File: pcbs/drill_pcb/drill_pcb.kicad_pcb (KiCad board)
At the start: 2 copper layers, 109 x 112 mm, 27 parts, among them J1 24V IN, J10 WEIGHT SENSOR, J11 STEPPER STORAGE, J2 DC MOTOR 24 V, J3 DC MOTOR UART, J4 ENCODER VERTICAL DRIVE, J5 LIMIT SENSOR TOP, J6 HEIGHT SENSOR, J7 STEPPER VERTICAL DRIVE, J8 ENCODER STORAGE, J9 LIMIT SENSOR BOTTOM, U1 ESP32-DevKitC, U2 LM3940

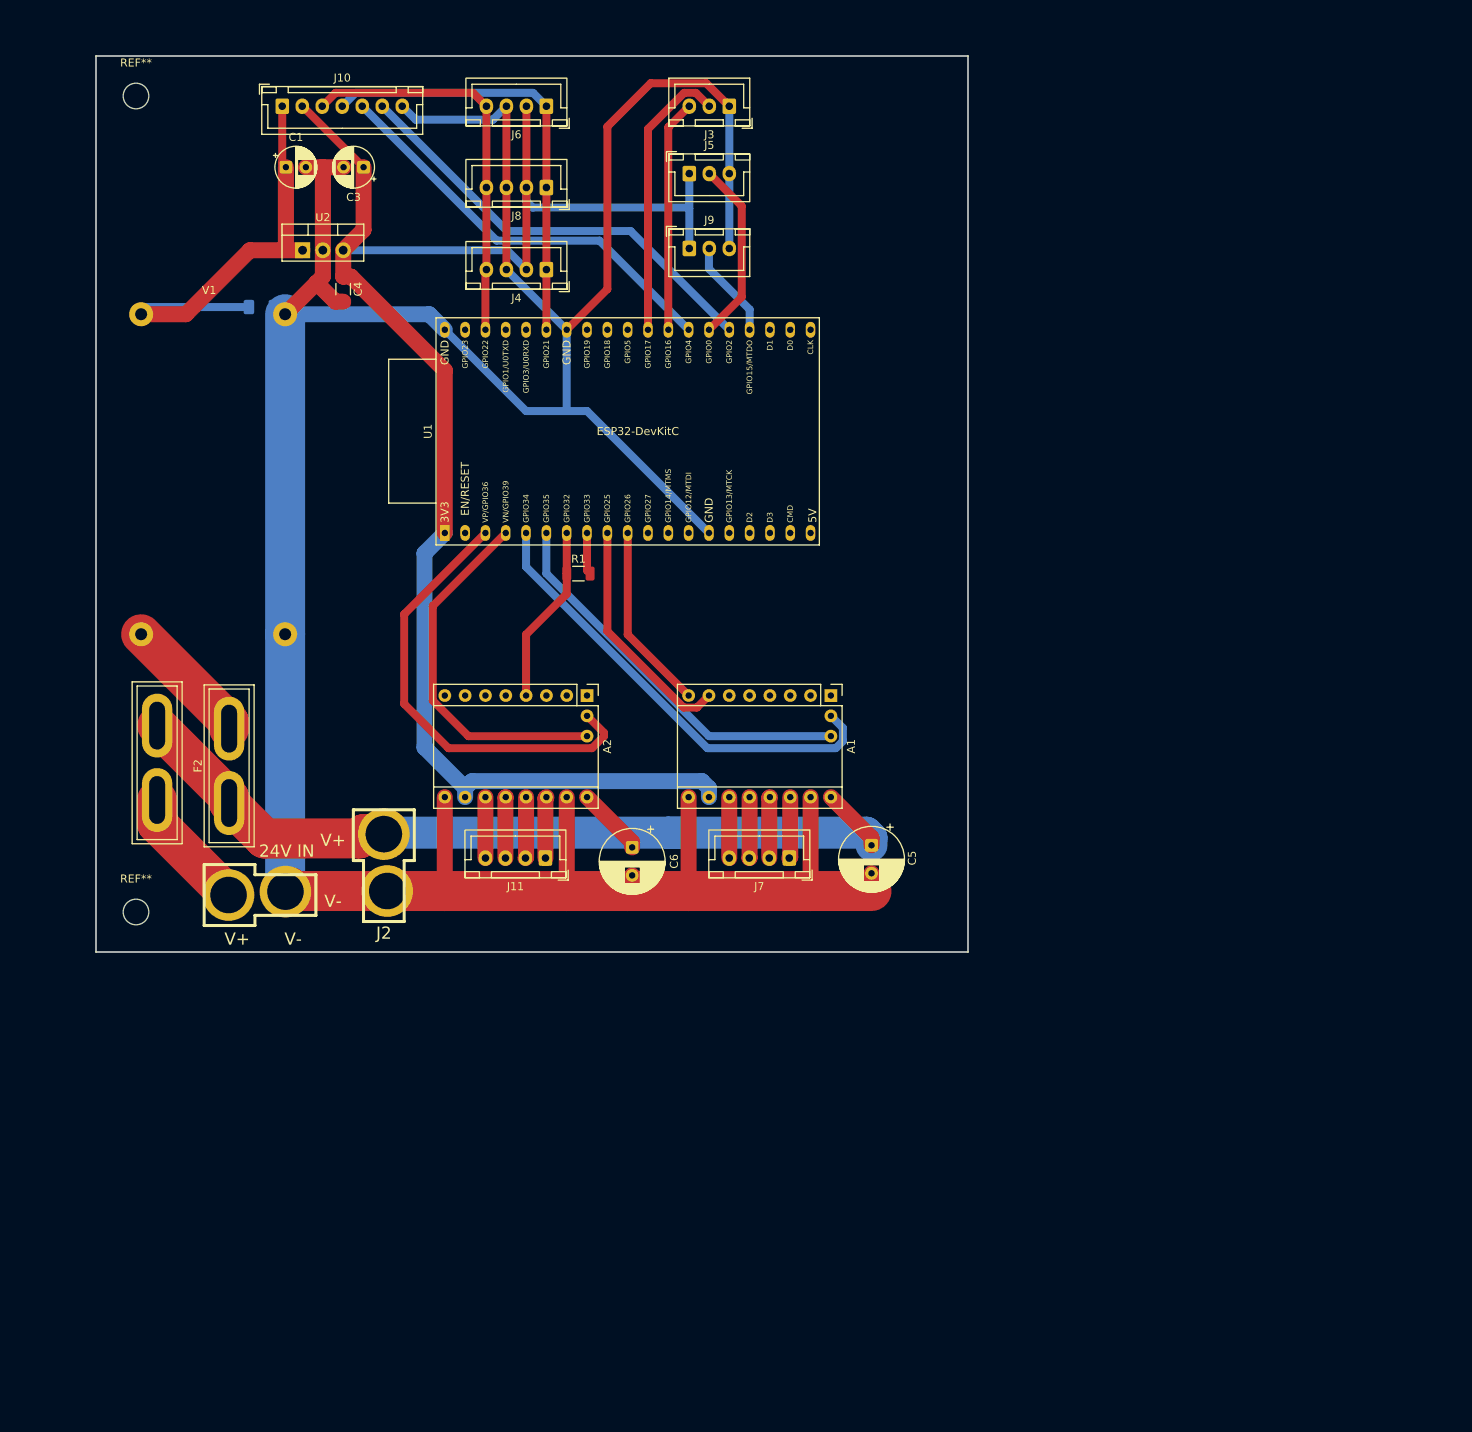
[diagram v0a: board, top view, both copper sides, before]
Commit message: PCB should be fully complete now. Somebody pls review it :(
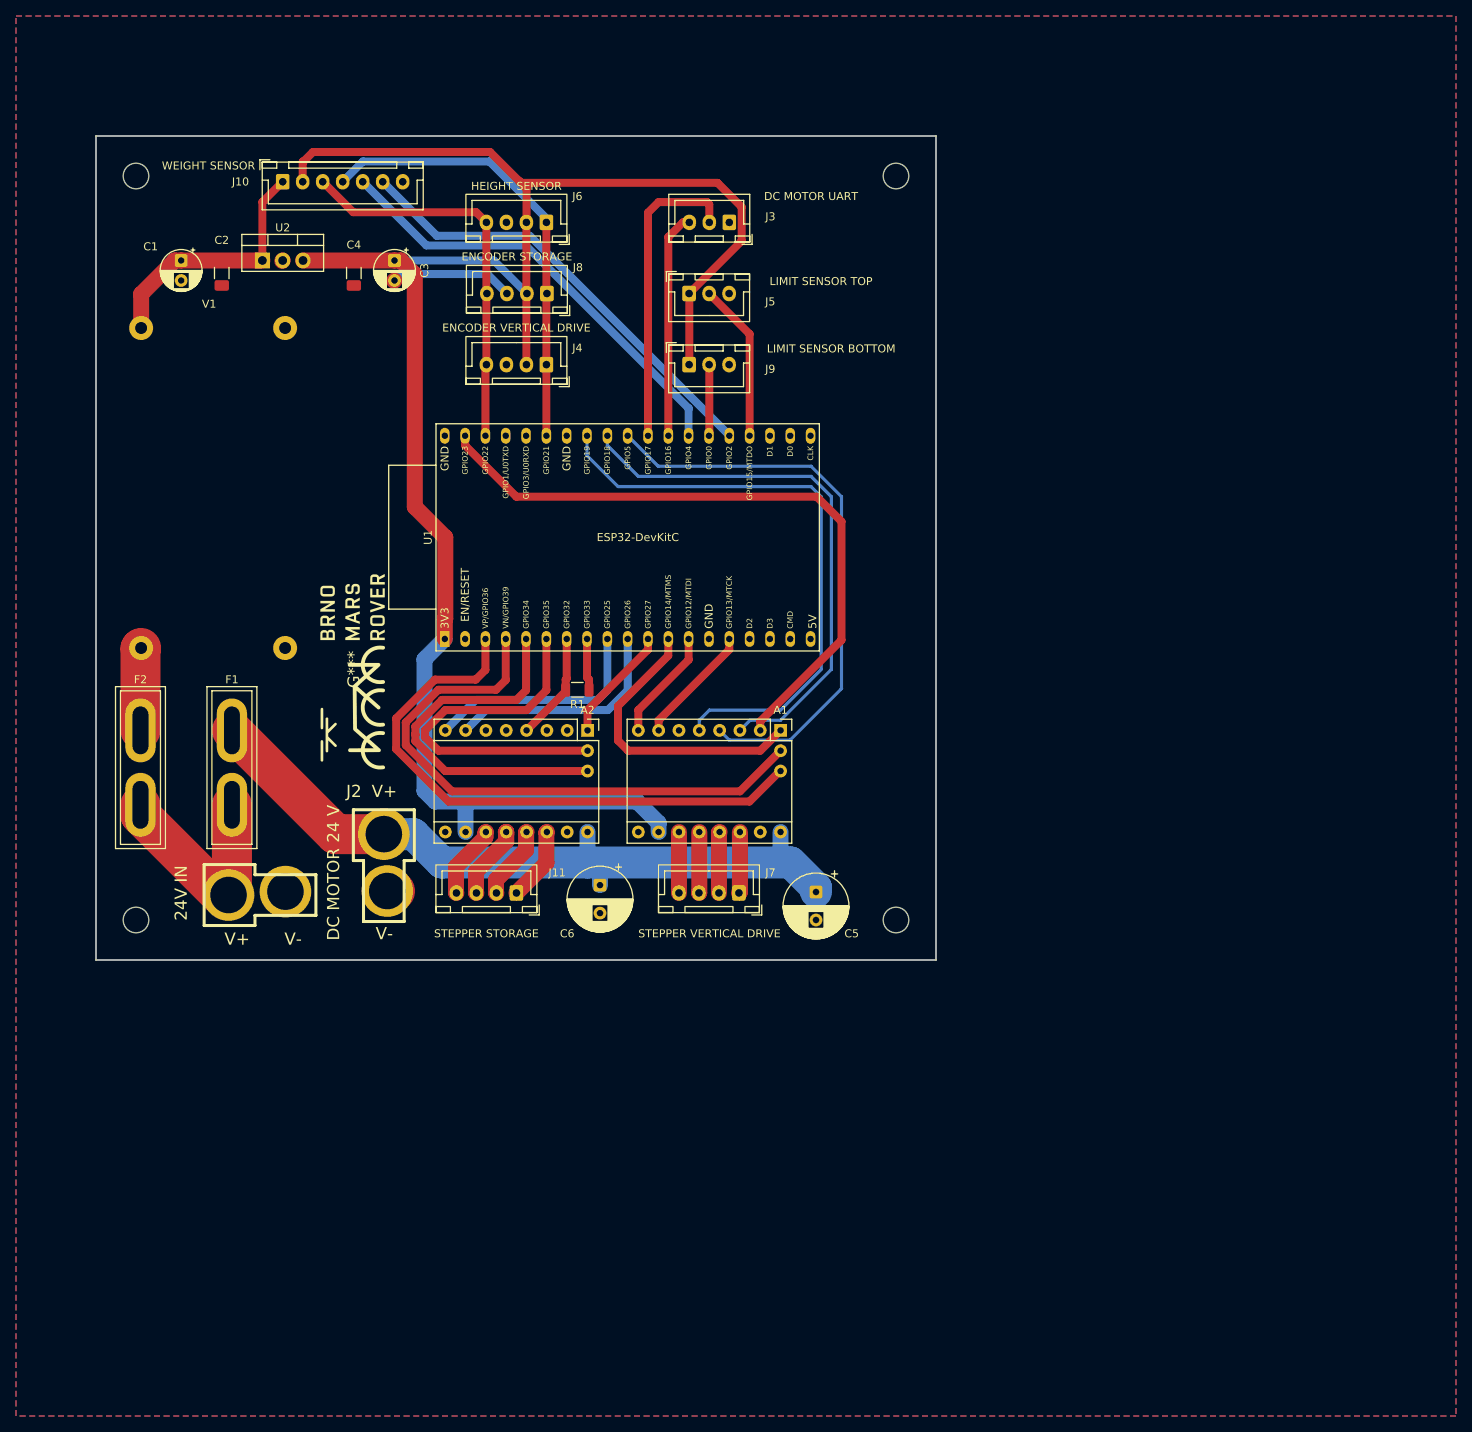
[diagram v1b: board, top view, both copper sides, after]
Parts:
- removed the REF** at (35.0, 137.0)
- removed the REF** at (35.0, 35.0)
- added G***: LOGO, logo:logo, F.Cu at (62.2, 106.7)
- added REF**: MountingHole_3.2mm_M3, MountingHole:MountingHole_3.2mm_M3, F.Cu at (35.0, 45.0)
- added REF**: MountingHole_3.2mm_M3, MountingHole:MountingHole_3.2mm_M3, F.Cu at (35.0, 138.0)
- added REF**: MountingHole_3.2mm_M3, MountingHole:MountingHole_3.2mm_M3, F.Cu at (130.0, 138.0)
- added REF**: MountingHole_3.2mm_M3, MountingHole:MountingHole_3.2mm_M3, F.Cu at (130.0, 45.0)
- C2: moved to F.Cu
- moved C1 17.5 mm to (40.6, 55.6), turned to -90 degrees
- moved J5 15.0 mm to (104.1, 59.7)
- moved R1 14.5 mm to (90.2, 109.2)
- moved J9 14.5 mm to (104.1, 68.6)
- moved J3 14.5 mm to (109.2, 50.8)
- moved J6 14.5 mm to (86.3, 50.8)
- moved J8 13.3 mm to (86.4, 59.7)
- moved U1 13.2 mm to (73.6, 102.9)
- moved C3 12.3 mm to (67.3, 55.6), turned to -90 degrees
- moved J4 11.9 mm to (86.3, 68.6)
- moved F2 11.1 mm to (35.6, 123.6)
- moved J10 9.44 mm to (53.3, 45.7)
- moved F1 9.37 mm to (47.0, 123.6)
- moved C5 9.07 mm to (120.0, 134.5)
- moved A1 7.65 mm to (115.6, 114.3)
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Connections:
- F2 pad 1: +24V -> Net-(J1-Pin_1)
- U1 pad 10: DRVR_VERT_DIR -> DRVR_STORAGE_STEP
- U1 pad 11: DRVR_VERT_ENABLE -> DRVR_STORAGE_ENABLE
- U1 pad 12: DRVR_STORAGE_ENABLE -> DRVR_VERT_ENABLE
- U1 pad 13: DRVR_STORAGE_DIR -> DRVR_VERT_DIR
- U1 pad 15: DRVR_STORAGE_STEP -> DRVR_VERT_STEP
- U1 pad 23: LIMIT_SENSOR_BOTTOM -> LIMIT_SENSOR_TOP
- U1 pad 25: LIMIT_SENSOR_TOP -> LIMIT_SENSOR_BOTTOM
- U1 pad 3: DRVR_STORAGE_0 -> DRVR_VERT_DIAG1
- U1 pad 4: DRVR_STORAGE_1 -> DRVR_VERT_DIAG0
- U1 pad 5: DRVR_VERT_DIAG0 -> DRVR_STORAGE_1
- U1 pad 6: DRVR_VERT_DIAG1 -> DRVR_STORAGE_0
- U1 pad 9: DRVR_VERT_STEP -> DRVR_STORAGE_DIR
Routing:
- net GND: track 416.0 -> 16.6 mm
- net VSPI_MOSI: track 0.00 -> 82.5 mm
- net VSPI_MISO: track 0.00 -> 74.6 mm
- net VSPI_CS1: track 0.00 -> 72.3 mm
- net VSPI_SCK: track 0.00 -> 68.0 mm
- net DRVR_VERT_ENABLE: track 0.00 -> 37.2 mm
- net +3.3V: track 208.1 -> 244.1 mm
- net DRVR_STORAGE_DIR: track 0.00 -> 28.7 mm
- net DRVR_STORAGE_STEP: track 0.00 -> 28.7 mm
- net DRVR_VERT_DIAG1: track 49.1 -> 73.7 mm
- net +24V: track 117.6 -> 93.6 mm
- net +5V: track 55.8 -> 32.0 mm
- net DRVR_VERT_DIAG0: track 57.4 -> 74.0 mm
- net DRVR_STORAGE_ENABLE: track 0.00 -> 14.6 mm
- net DRVR_VERT_STEP: track 29.6 -> 15.1 mm
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- added copper zone on B.Cu, net GND
- added copper zone on F.Cu, net GND
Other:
- board size 109 x 112 mm -> 105 x 103 mm
